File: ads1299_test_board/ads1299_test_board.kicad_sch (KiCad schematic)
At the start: 0 parts

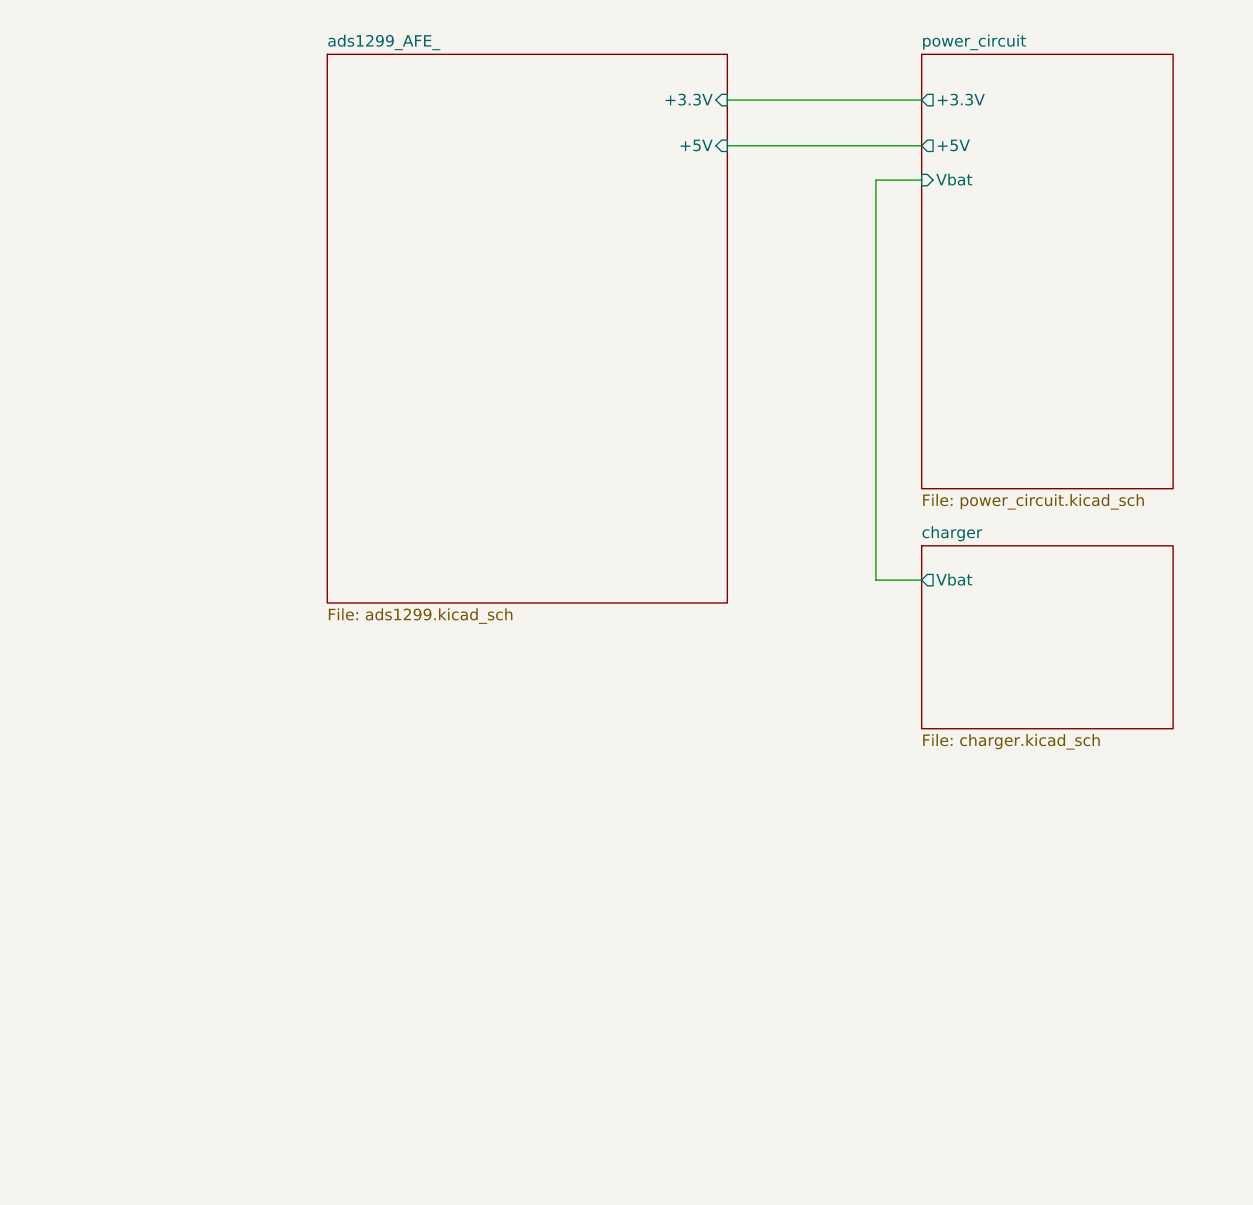
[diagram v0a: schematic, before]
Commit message: usb, esp32 s3 wroom 1
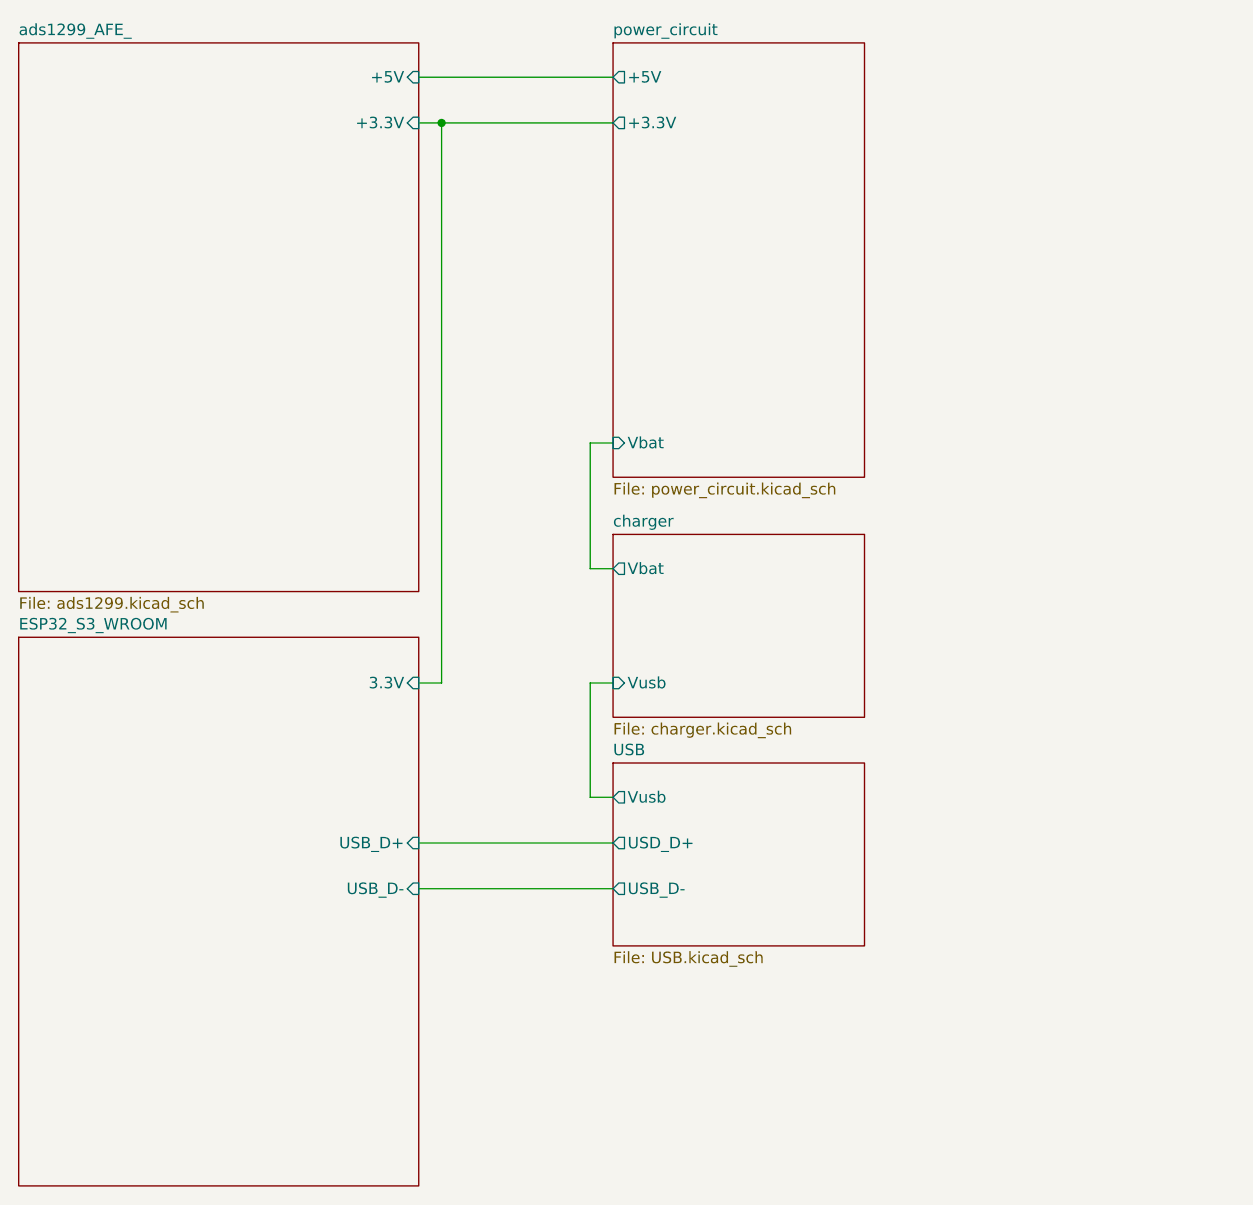
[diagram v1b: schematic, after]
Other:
- added sheet ESP32_S3_WROOM (ESP32_S3_WROOM.kicad_sch)
- added sheet USB (USB.kicad_sch)
- sheet charger ports: added Vusb; removed none
